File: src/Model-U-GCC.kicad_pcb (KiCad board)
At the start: 2 copper layers, 20 x 13.5 mm, 6 parts, among them J1 USB_C_Receptacle, J2 Conn_01x04, J3 Conn_01x04

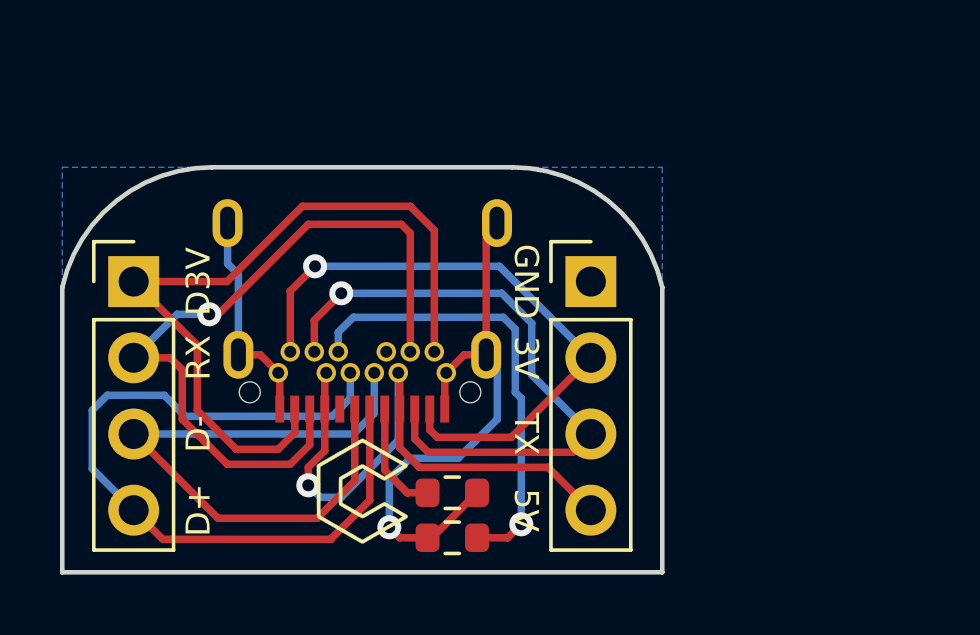
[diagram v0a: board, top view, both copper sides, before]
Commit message: Model U GCC v1
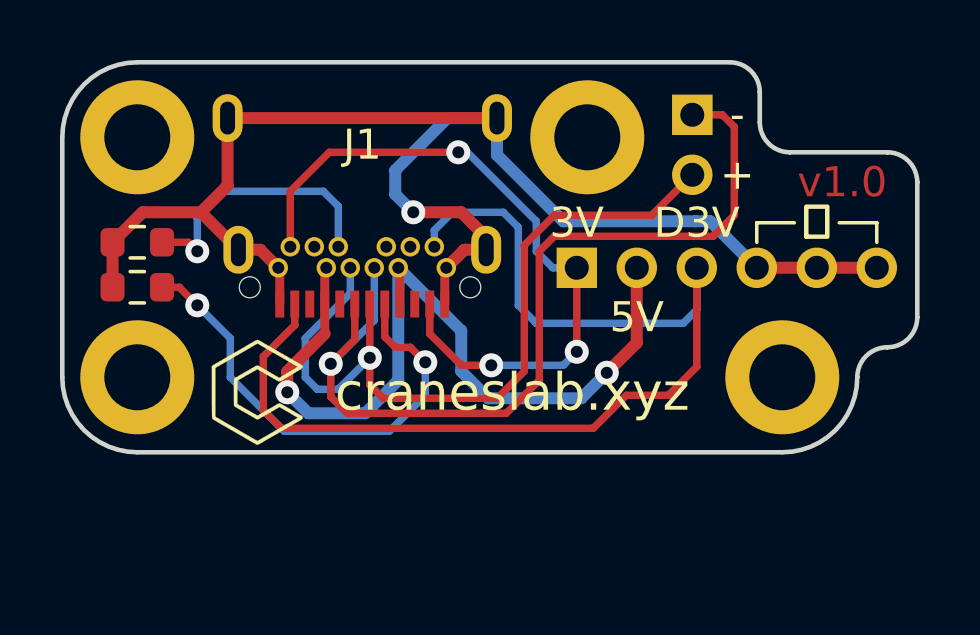
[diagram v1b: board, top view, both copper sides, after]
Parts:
- added REF**: MountingHole_2.2mm_M2_DIN965_Pad, MountingHole:MountingHole_2.2mm_M2_DIN965_Pad, F.Cu at (14.0, 7.00)
- added REF**: MountingHole_2.2mm_M2_DIN965_Pad, MountingHole:MountingHole_2.2mm_M2_DIN965_Pad, F.Cu at (-7.50, 7.00)
- added REF**: MountingHole_2.2mm_M2_DIN965_Pad, MountingHole:MountingHole_2.2mm_M2_DIN965_Pad, F.Cu at (7.50, -1.00)
- added REF**: MountingHole_2.2mm_M2_DIN965_Pad, MountingHole:MountingHole_2.2mm_M2_DIN965_Pad, F.Cu at (-7.50, -1.00)
- J2: value Conn_01x04 -> Conn_01x06; footprint Model_S:PinHeader_1x04_P2.54mm_Vertical -> Connector_PinHeader_2.00mm:PinHeader_1x06_P2.00mm_Vertical
- J3: value Conn_01x04 -> Conn_01x02; footprint Model_S:PinHeader_1x04_P2.54mm_Vertical -> Connector_PinHeader_2.00mm:PinHeader_1x02_P2.00mm_Vertical
- R1, R2: value R -> 5.1k
- moved J2 14.8 mm to (7.15, 3.35), turned to 90 degrees
- moved R2 14.4 mm to (-7.50, 2.50)
- moved R1 12.5 mm to (-7.50, 4.00), turned to 0 degrees
- moved J3 6.51 mm to (11.0, -1.75)
- moved G*** 4.81 mm to (-3.50, 7.50)
- moved J1 3.50 mm to (0.00, -3.50)
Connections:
- J1 pad A10: RX- -> Net-(J1-PadA10)
- J1 pad A3: TX- -> Net-(J1-PadA3)
- J1 pad B10: RX- -> Net-(J1-PadB10)
- J1 pad B3: TX- -> Net-(J1-PadB3)
- J2 pad 1: D3V -> 3V3
- J2 pad 2: RX- -> VBUS
- J2 pad 3: D- -> D3V
- J2 pad 4: D+ -> GND
- J3 pad 1: GND -> D-
- J3 pad 2: 3V3 -> D+
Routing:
- net RX-: track 24.9 -> 0.00 mm, vias 1 -> 0
- net GND: track 26.7 -> 49.1 mm
- net TX-: track 20.9 -> 0.00 mm, vias 1 -> 0
- net D3V: track 25.4 -> 37.0 mm
- net Net-(J1-PadA5): track 4.48 -> 15.9 mm, vias 0 -> 2
- net D-: track 21.1 -> 30.7 mm, vias 0 -> 1
- net VBUS: track 20.0 -> 27.9 mm, vias 1 -> 2
- net Net-(J1-PadB5): track 15.2 -> 9.03 mm
- net 3V3: track 20.9 -> 23.4 mm, vias 1 -> 3
- net D+: track 25.9 -> 26.2 mm, vias 0 -> 1
- removed copper zone on B.Cu, net GND
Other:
- board size 20 x 13.5 mm -> 28.5 x 13 mm
- board text added: "+"
- board text added: "-"
- board text added: "JLCJLCJLCJLC"
- board text added: "v1.0"
- board text added: "⏚"
- board text removed: "D+"
- board text removed: "D-"
- board text removed: "GND"
- board text removed: "RX"
- board text removed: "TX"
- board text removed: "v3"
